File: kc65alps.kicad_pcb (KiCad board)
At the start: 2 copper layers, 304.8 x 95.3 mm, 160 parts, among them J1 Conn_01x04, J2 AVR-ISP-6, U1 ATmega32U4-AU, Y1 16MHz

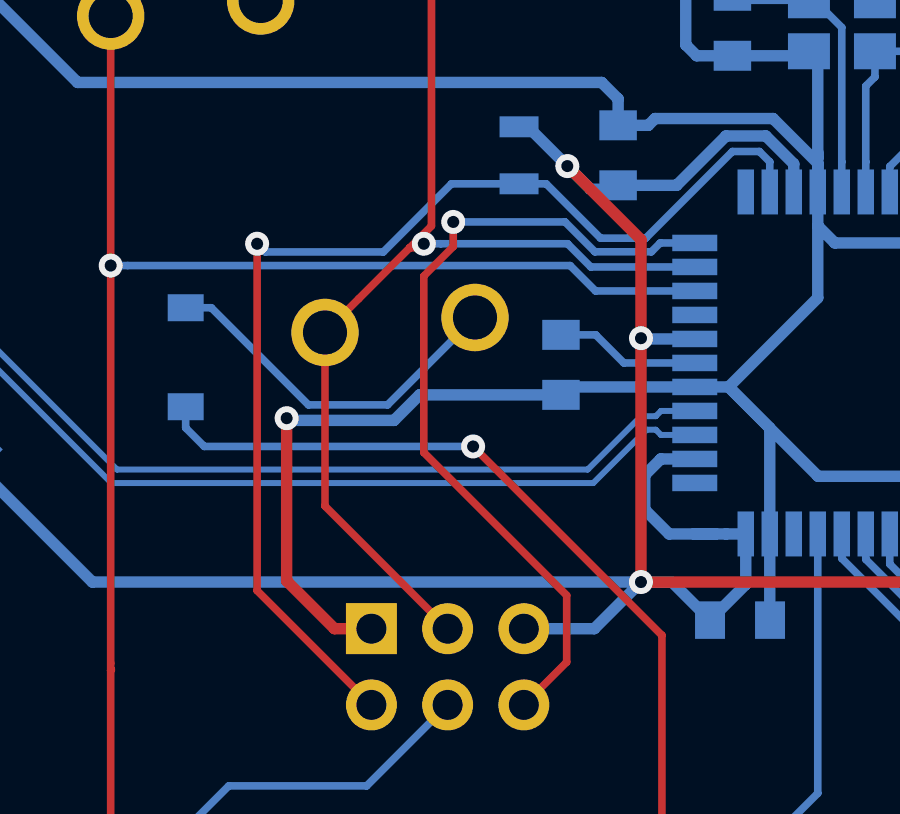
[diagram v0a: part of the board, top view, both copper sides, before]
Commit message: PCB update
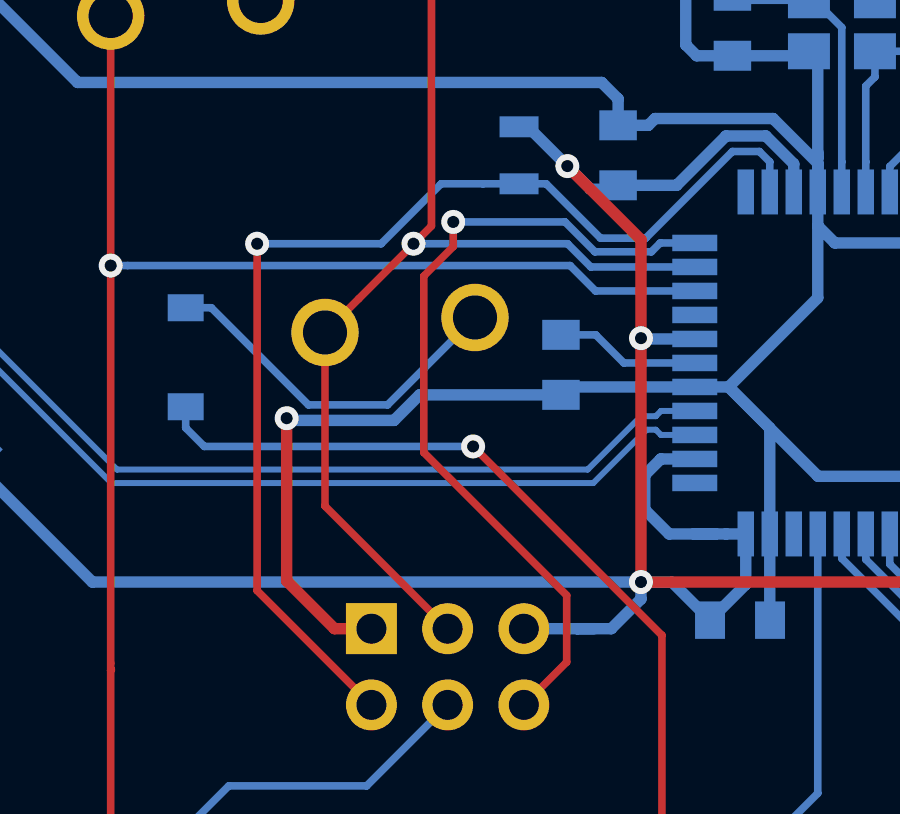
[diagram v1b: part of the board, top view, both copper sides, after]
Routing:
- net +5V: track 111.6 -> 112.5 mm
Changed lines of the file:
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@@
     (thickness 1.6)
     (drawings 8)
-    (tracks 635)
+    (tracks 636)
     (zones 0)
     (modules 160)
@@
   (segment (start 30.226 150.368) (end 26.121528 146.263528) (width 0.381) (layer B.Cu) (net 5))
   (segment (start 48.514 150.368) (end 30.226 150.368) (width 0.381) (layer B.Cu) (net 5))
-  (segment (start 46.95825 151.92375) (end 48.514 150.368) (width 0.381) (layer B.Cu) (net 5))
-  (segment (start 44.60875 151.92375) (end 46.95825 151.92375) (width 0.381) (layer B.Cu) (net 5))
   (segment (start 52.676859 135.49949) (end 51.347642 135.49949) (width 0.381) (layer B.Cu) (net 5))
   (segment (start 53.607 137.3655) (end 53.607 136.429631) (width 0.381) (layer B.Cu) (net 5))
@@
   (segment (start 61.468 150.368) (end 64.135 147.701) (width 0.381) (layer F.Cu) (net 5))
   (segment (start 48.514 150.368) (end 61.468 150.368) (width 0.381) (layer F.Cu) (net 5))
+  (segment (start 47.523935 151.92375) (end 46.38675 151.92375) (width 0.381) (layer B.Cu) (net 5))
+  (segment (start 48.514 150.933685) (end 47.523935 151.92375) (width 0.381) (layer B.Cu) (net 5))
+  (segment (start 48.514 150.368) (end 48.514 150.933685) (width 0.381) (layer B.Cu) (net 5))
+  (segment (start 44.60875 151.92375) (end 46.38675 151.92375) (width 0.381) (layer B.Cu) (net 5))
+  (segment (start 46.38675 151.92375) (end 46.95825 151.92375) (width 0.381) (layer B.Cu) (net 5))
   (segment (start 38.1 88.16875) (end 57.15 88.16875) (width 0.254) (layer B.Cu) (net 6))
   (segment (start 57.15 88.16875) (end 58.004 88.16875) (width 0.254) (layer B.Cu) (net 6))
@@
   (segment (start 24.92375 123.845001) (end 24.92375 122.87) (width 0.2) (layer B.Cu) (net 81))
   (segment (start 50.307 144.6655) (end 49.181999 144.6655) (width 0.2) (layer B.Cu) (net 81))
-  (segment (start 42.196788 137.094) (end 39.926048 139.36474) (width 0.254) (layer B.Cu) (net 82))
-  (segment (start 44.45 137.094) (end 42.196788 137.094) (width 0.254) (layer B.Cu) (net 82))
   (via (at 35.71875 139.09175) (size 0.8) (drill 0.4) (layers F.Cu B.Cu) (net 82))
-  (segment (start 39.926048 139.36474) (end 35.99174 139.36474) (width 0.254) (layer B.Cu) (net 82))
-  (segment (start 35.99174 139.36474) (end 35.71875 139.09175) (width 0.254) (layer B.Cu) (net 82))
   (segment (start 35.71875 150.65375) (end 39.52875 154.46375) (width 0.254) (layer F.Cu) (net 82))
   (segment (start 35.71875 139.09175) (end 35.71875 150.65375) (width 0.254) (layer F.Cu) (net 82))
@@
   (segment (start 47.16625 138.90625) (end 48.10125 138.90625) (width 0.254) (layer B.Cu) (net 82))
   (segment (start 48.10125 138.90625) (end 48.41875 138.90625) (width 0.254) (layer B.Cu) (net 82))
+  (segment (start 41.851913 137.094) (end 43.246 137.094) (width 0.254) (layer B.Cu) (net 82))
+  (segment (start 39.854163 139.09175) (end 41.851913 137.094) (width 0.254) (layer B.Cu) (net 82))
+  (segment (start 35.71875 139.09175) (end 39.854163 139.09175) (width 0.254) (layer B.Cu) (net 82))
+  (segment (start 44.45 137.094) (end 43.246 137.094) (width 0.254) (layer B.Cu) (net 82))
   (via (at 42.256249 138.36475) (size 0.8) (drill 0.4) (layers F.Cu B.Cu) (net 83))
   (segment (start 42.427999 138.5365) (end 42.256249 138.36475) (width 0.254) (layer B.Cu) (net 83))
@@
   (segment (start 41.529249 88.495751) (end 41.529249 138.502001) (width 0.254) (layer F.Cu) (net 86))
   (segment (start 45.125 84.9) (end 41.529249 88.495751) (width 0.254) (layer F.Cu) (net 86))
-  (via (at 41.275 139.09175) (size 0.8) (drill 0.4) (layers F.Cu B.Cu) (net 86))
-  (segment (start 41.138625 139.228125) (end 41.275 139.09175) (width 0.254) (layer F.Cu) (net 86))
-  (segment (start 40.803125 139.228125) (end 41.138625 139.228125) (width 0.254) (layer F.Cu) (net 86))
   (segment (start 40.803125 139.228125) (end 39.106249 140.925001) (width 0.254) (layer F.Cu) (net 86))
   (segment (start 41.529249 138.502001) (end 40.803125 139.228125) (width 0.254) (layer F.Cu) (net 86))
   (segment (start 37.98125 147.83625) (end 37.98125 142.05) (width 0.254) (layer F.Cu) (net 86))
   (segment (start 42.06875 151.92375) (end 37.98125 147.83625) (width 0.254) (layer F.Cu) (net 86))
-  (segment (start 41.840685 139.09175) (end 41.275 139.09175) (width 0.254) (layer B.Cu) (net 86))
-  (segment (start 46.067618 139.091751) (end 41.840685 139.09175) (width 0.254) (layer B.Cu) (net 86))
+  (segment (start 41.275 139.09175) (end 40.930125 139.09175) (width 0.254) (layer B.Cu) (net 86))
+  (segment (start 46.067618 139.091751) (end 41.275 139.09175) (width 0.254) (layer B.Cu) (net 86))
   (segment (start 46.841367 139.8655) (end 46.067618 139.091751) (width 0.254) (layer B.Cu) (net 86))
+  (via (at 40.930125 139.09175) (size 0.8) (drill 0.4) (layers F.Cu B.Cu) (net 86))
   (segment (start 50.307 139.8655) (end 46.841367 139.8655) (width 0.254) (layer B.Cu) (net 86))
   (segment (start 54.65 94.425) (end 64.175 84.9) (width 0.254) (layer F.Cu) (net 87))
